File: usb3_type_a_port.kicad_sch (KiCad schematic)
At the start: 13 parts, among them J4 USB3_A, U14 TPD4E02B04, U15 ESD122, U16 TPS2557

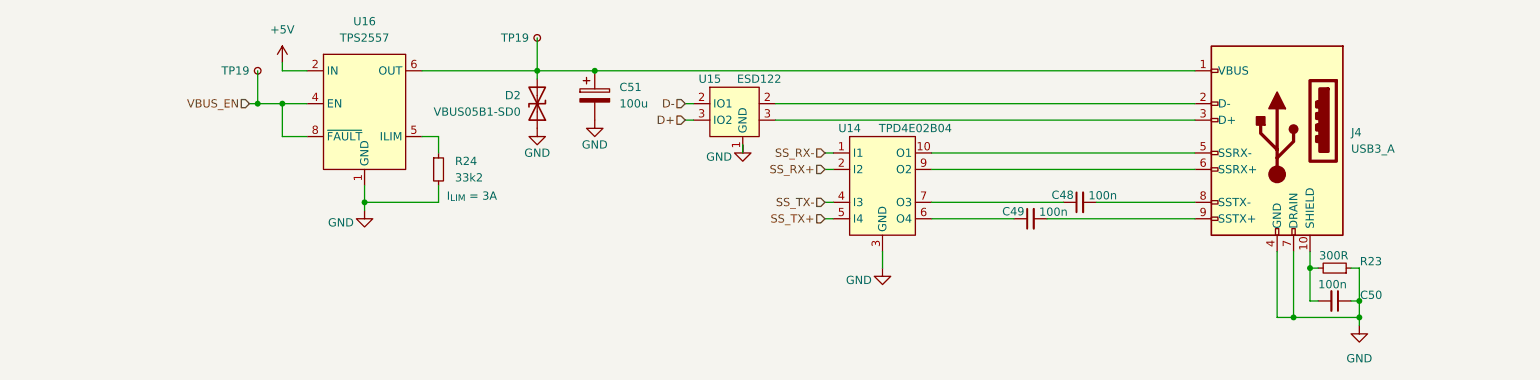
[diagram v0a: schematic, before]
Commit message: layout
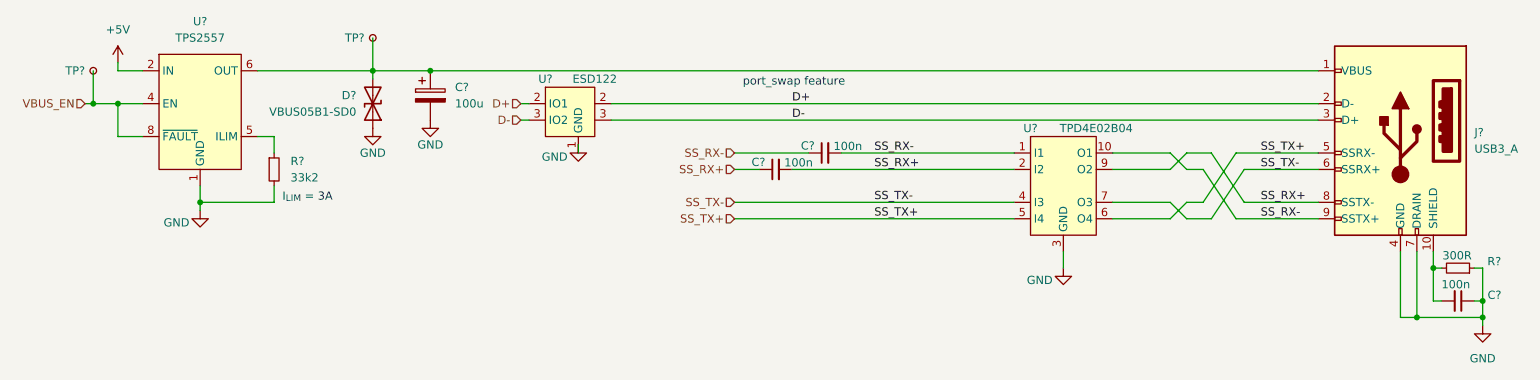
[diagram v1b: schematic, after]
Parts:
- C?: renamed from C48; footprint Resistor_SMD:R_0402_1005Metric -> Capacitor_SMD:C_0402_1005Metric; LCSC (none) -> C386075; MPN (none) -> TMK105B7104KVHF
- C?: renamed from C49; footprint Resistor_SMD:R_0402_1005Metric -> Capacitor_SMD:C_0402_1005Metric; LCSC (none) -> C386075; MPN (none) -> TMK105B7104KVHF
- C?: renamed from C50; footprint (none) -> Capacitor_SMD:C_0402_1005Metric; LCSC (none) -> C386075; MPN (none) -> TMK105B7104KVHF
- C?: renamed from C51; footprint (none) -> Capacitor_SMD:CP_Elec_8x10.5; LCSC (none) -> C5162347; MPN (none) -> CS1H101M-CRF10
- D?: renamed from D2; LCSC (none) -> C2859524; MPN (none) -> VBUS05B1-SD0-G4-08
- J?: renamed from J4; footprint (none) -> Connector_USB:USB3_A-TH_U231-091N-4BLCC14-S-5; LCSC (none) -> C388644; MPN (none) -> U231-091N-4BLCC14-S5
- R?: renamed from R23; footprint (none) -> Resistor_SMD:R_0402_1005Metric; LCSC (none) -> C25102; MPN (none) -> 0402WGF3000TCE
- R?: renamed from R24; footprint (none) -> Resistor_SMD:R_0402_1005Metric; LCSC (none) -> C122548; MPN (none) -> 0402WGF3322TCE
- U?: renamed from U14; LCSC (none) -> C106794; MPN (none) -> TPD4E02B04DQAR
- U?: renamed from U15; LCSC (none) -> C544474; MPN (none) -> ESD122DMXR
- U?: renamed from U16; LCSC (none) -> C130056; MPN (none) -> TPS2557DRBR
- renumbered TP19 to TP?
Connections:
- net D+: now also J?.2 (D-), U?.2 (IO1); no longer U?.3 (IO2)
- net D-: now also J?.3 (D+), U?.3 (IO2); no longer U?.2 (IO1)
- net SS_RX+: now also C?.1, C?.2, J?.8 (SSTX-), U?.9 (O2)
- net SS_RX-: now also C?.1, C?.2, J?.9 (SSTX+), U?.10 (O1)
- net SS_TX+: now also J?.5 (SSRX-), U?.6 (O4)
- net SS_TX-: now also J?.6 (SSRX+), U?.7 (O3)
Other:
- note added: "port_swap feature"
- moved on the sheet: C?, D?, J?, R?, TP?, U?
